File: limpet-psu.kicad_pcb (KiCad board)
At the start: 2 copper layers, 27 x 18 mm, 16 parts, among them J1 USB_C_Receptacle_HRO_TYPE-C-3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, U1 RT6154AGQW

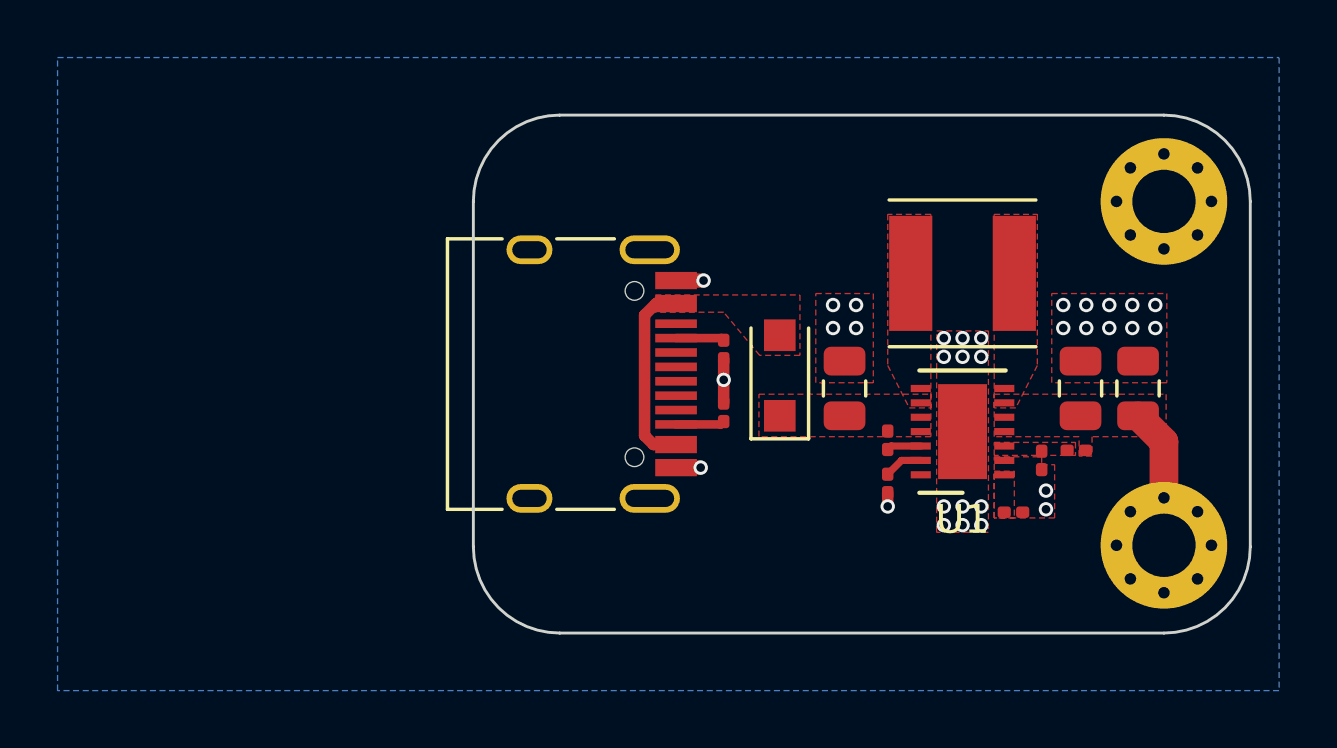
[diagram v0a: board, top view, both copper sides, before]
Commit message: output
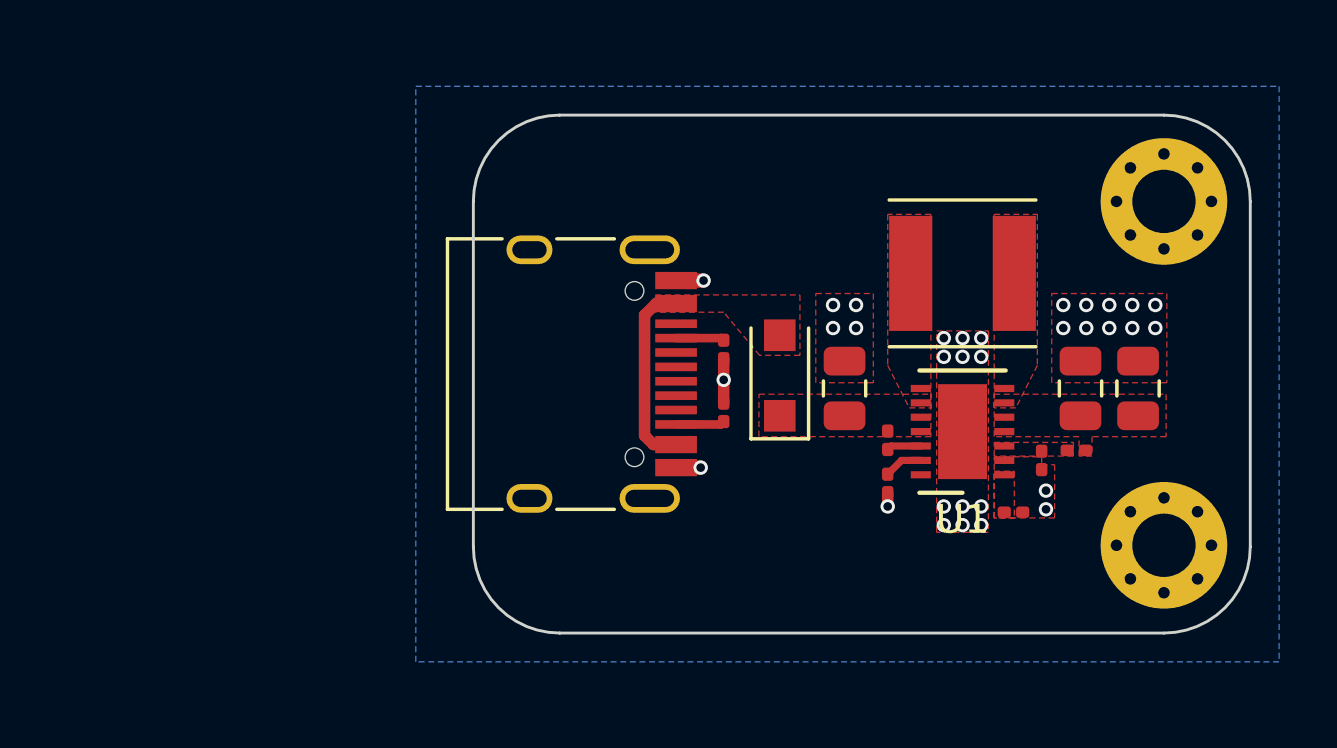
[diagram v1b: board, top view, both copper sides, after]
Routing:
- net +3V3: track 5.12 -> 0.25 mm
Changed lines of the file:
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@@
   (via (at 195.5 77.4) (size 0.5) (drill 0.3) (layers "F.Cu" "B.Cu") (free) (net 1))
   (segment (start 204.1 80.45) (end 204.275 80.625) (width 0.4) (layer "F.Cu") (net 4))
-  (segment (start 207 84.95) (end 207 81.35) (width 1) (layer "F.Cu") (net 4))
-  (segment (start 207 81.35) (end 206.1 80.45) (width 1) (layer "F.Cu") (net 4))
   (segment (start 188.95 81.139004) (end 188.95 76.95) (width 0.4) (layer "F.Cu") (net 5))
   (segment (start 190.045 81.45) (end 189.260996 81.45) (width 0.4) (layer "F.Cu") (net 5))
@@
     (polygon
       (pts
-        (xy 203.925 81.825)
-        (xy 201.1 81.825)
+        (xy 203.85 81.85)
+        (xy 201.1 81.85)
         (xy 201.1 81.375)
-        (xy 203.925 81.375)
+        (xy 203.85 81.375)
       )
     )
@@
     (polygon
       (pts
-        (xy 211 90)
-        (xy 168.55 90)
-        (xy 168.55 68)
-        (xy 211 68)
+        (xy 211 89)
+        (xy 181 89)
+        (xy 181 69)
+        (xy 211 69)
       )
     )
